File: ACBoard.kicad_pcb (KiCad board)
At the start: 2 copper layers, 61.6 x 55.2 mm, 32 parts, among them J1 Conn_02x20_Odd_Even, J2 Conn_02x20_Odd_Even, J3 Conn_01x02_Male, J4 Conn_01x02_Female, J5 Conn_01x02_Female, T1 CSE185L, U1 TLP561, U2 TLP561, U3 ADS7822U

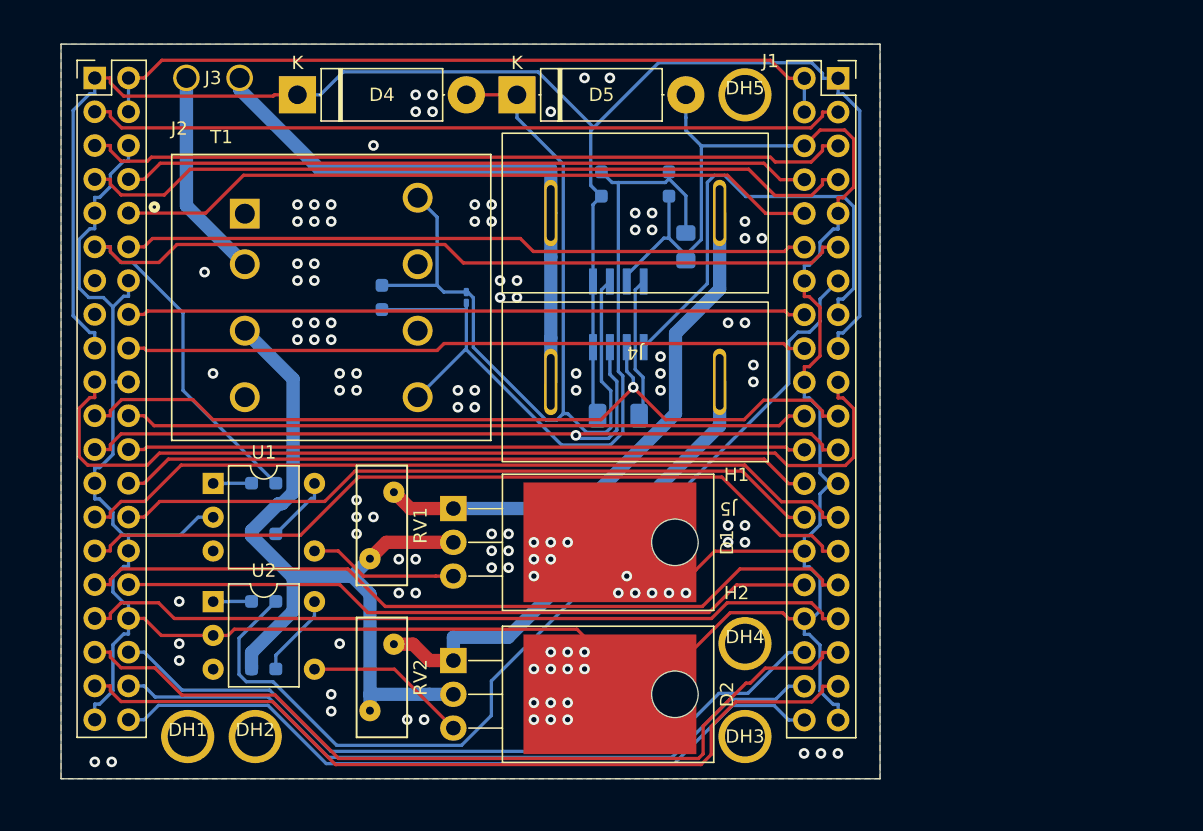
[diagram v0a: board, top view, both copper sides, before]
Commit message: AnoTation
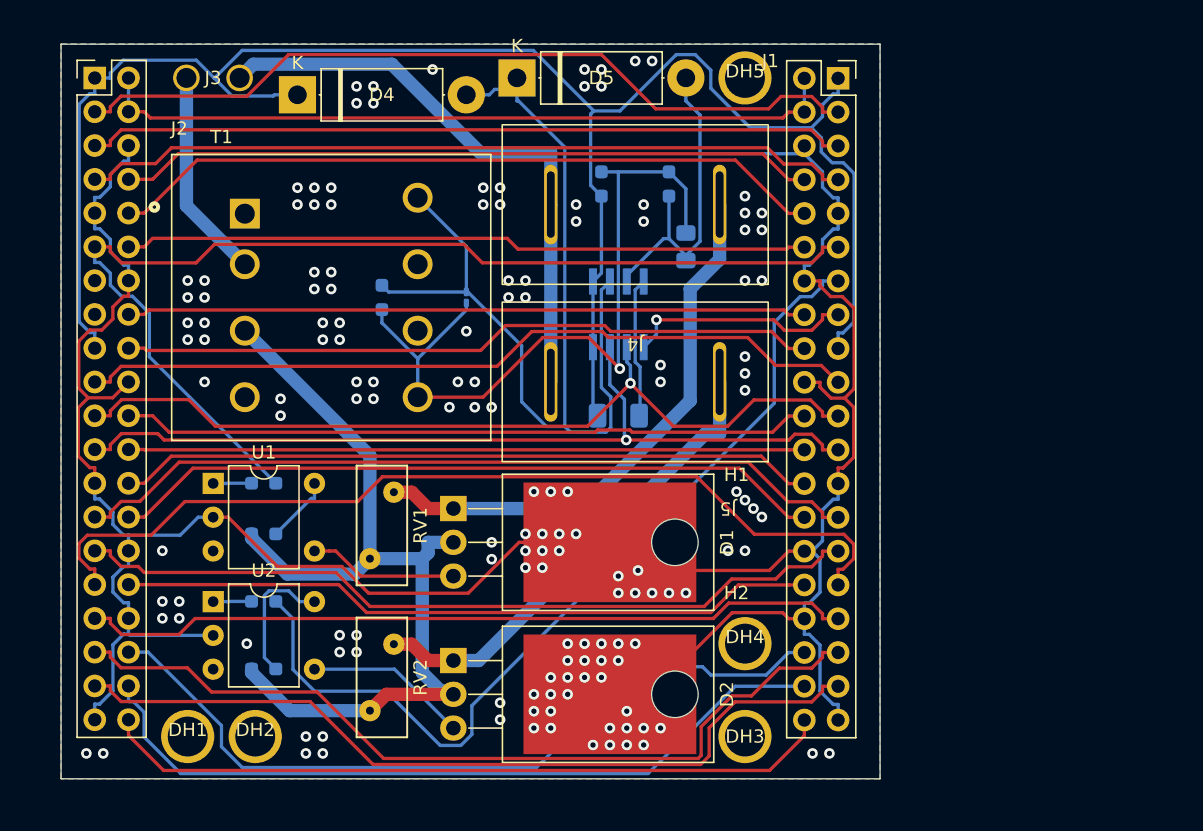
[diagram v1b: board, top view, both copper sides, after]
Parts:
- moved D5 1.27 mm to (191.8, 19.1)
- moved DH5 1.27 mm to (208.9, 19.1)
- moved J4 0.64 mm to (200.7, 28.6)
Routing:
- net /GPIO22: track 35.4 -> 17.1 mm, vias 0 -> 1
- net /GPIO10: track 72.2 -> 59.3 mm
- net +3V3: track 128.6 -> 139.0 mm
- net /USB_DM: track 59.7 -> 70.0 mm
- net VAC: track 61.1 -> 67.8 mm
- net /GPIO27: track 72.7 -> 68.5 mm
- net Net-(R4-Pad1): track 6.27 -> 10.1 mm
- net GND: track 224.4 -> 228.2 mm, vias 114 -> 146
- net Net-(D3-Pad2): track 72.5 -> 76.3 mm
- net /GPIO2: track 57.3 -> 60.7 mm
- net Net-(C1-Pad1): track 59.7 -> 56.5 mm, vias 0 -> 1
- net /DIN: track 55.3 -> 58.0 mm
- net /GPIO16: track 57.0 -> 59.5 mm
- net /GPIO11: track 67.3 -> 65.2 mm
- net /GPIO5: track 60.9 -> 59.8 mm
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
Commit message: data5
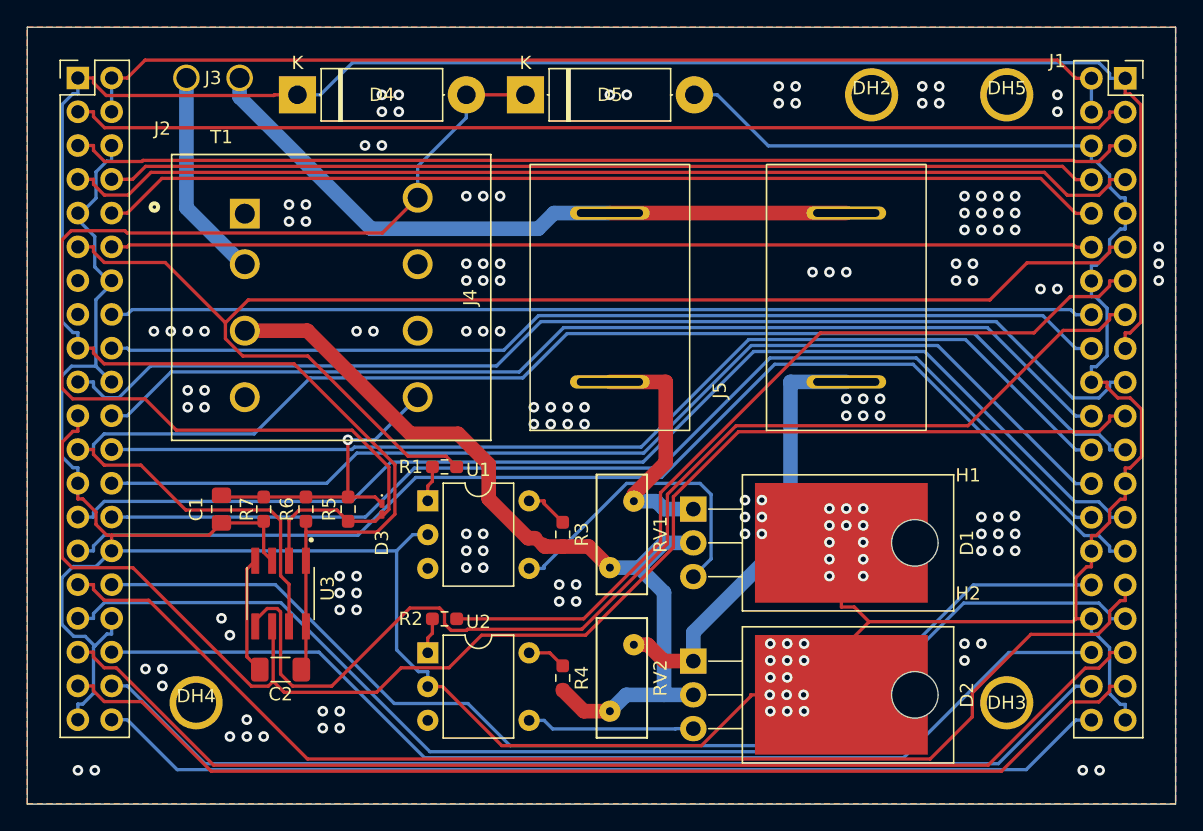
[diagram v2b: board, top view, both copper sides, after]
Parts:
- removed DH1: Drill, locallib:Drill
- C1, C2, D3, R1, R2, R3, R4, R5, R6, R7, U3: moved to F.Cu
- moved DH2 66.9 mm to (218.4, 20.3)
- moved DH4 41.5 mm to (167.6, 66.0)
- moved C1 40.1 mm to (169.5, 51.5)
- moved R7 39.1 mm to (172.7, 51.5)
- moved R6 33.0 mm to (175.9, 51.5)
- moved U3 33.0 mm to (174.0, 57.8)
- moved C2 31.8 mm to (174.0, 63.5), turned to 180 degrees
- moved R4 22.5 mm to (195.2, 64.2), turned to -90 degrees
- moved R3 22.5 mm to (195.2, 53.4), turned to -90 degrees
- moved J1 21.6 mm to (237.5, 19.1)
- moved DH3 19.8 mm to (228.6, 66.0)
- moved DH5 19.7 mm to (228.6, 20.3)
- moved RV1 18.1 mm to (198.8, 55.9)
- moved D1 18.0 mm to (205.0, 51.5)
- moved D2 18.0 mm to (205.0, 62.9)
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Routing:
- net /GPIO22: track 17.1 -> 87.2 mm, vias 1 -> 0
- net /GPIO11: track 65.2 -> 112.3 mm, vias 1 -> 0
- net /GPIO9: track 64.5 -> 111.0 mm, vias 1 -> 0
- net +3V3: track 139.0 -> 174.7 mm
- net GND: track 228.2 -> 263.8 mm, vias 146 -> 159
- net Net-(C1-Pad1): track 56.5 -> 23.2 mm
- net /GPIO12: track 52.6 -> 83.7 mm
- net /USB_DP: track 58.3 -> 89.4 mm
- net /GPIO5: track 59.8 -> 90.8 mm
- net /CE1: track 52.5 -> 82.3 mm
- net /EEPROM_SDA: track 59.8 -> 89.5 mm
- net /EEPROM_SCL: track 53.9 -> 83.6 mm
- net /CE0: track 50.8 -> 80.5 mm
- net /GPIO25: track 52.0 -> 79.2 mm
- net /GPIO10: track 59.3 -> 84.9 mm
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- added copper zone on B.Cu, net GNDA
- added copper zone on F.Cu, net GNDA
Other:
- board size 61.6 x 55.2 mm -> 86.4 x 58.4 mm
